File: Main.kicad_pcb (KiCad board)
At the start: 2 copper layers, 170.2 x 137.2 mm, 60 parts, among them J1 Conn_01x01_Male, J2 Conn_01x06_Male, J3 Conn_01x04_Male, J4 Conn_01x01_Male, J5 Conn_01x05_Male, J6 Conn_01x03, J7 Conn_01x03, J8 Conn_01x06, J9 Conn_01x05_Male, Q1 CSD17307Q5A, Q2 CSD17307Q5A, U1 LM4120-CustomSymbols, U2 LTC2942, U3 LM393, U4 TPS2557, U5 LM393, U6 TPS2557, U7 SN74LVC2G08

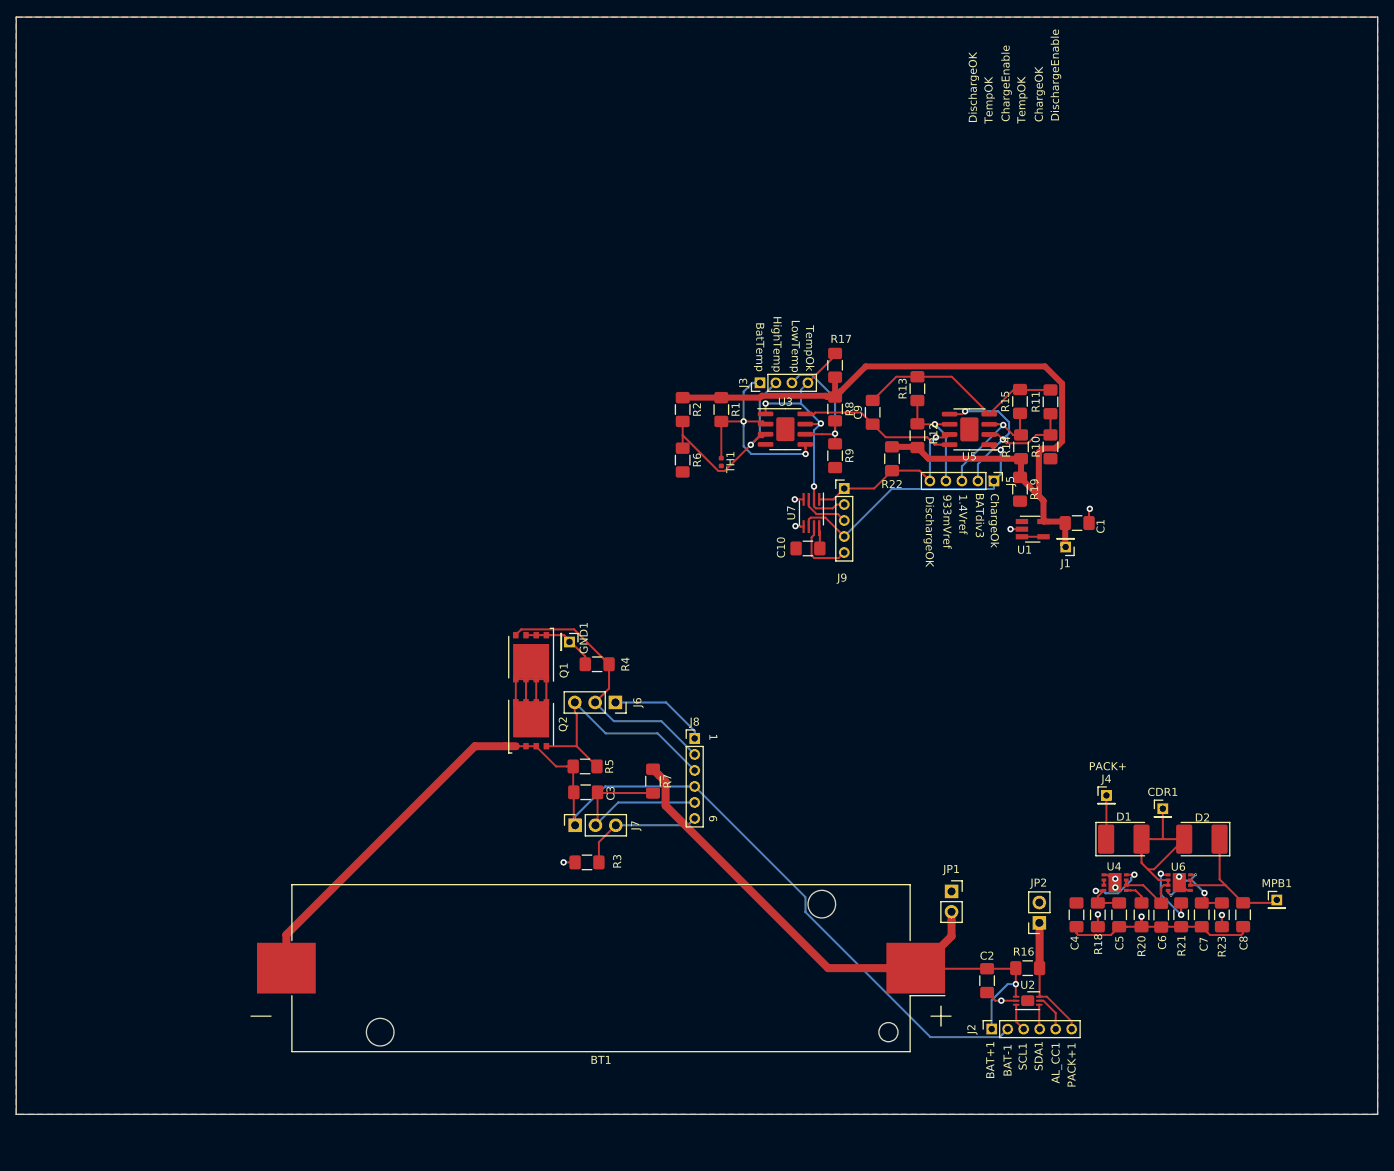
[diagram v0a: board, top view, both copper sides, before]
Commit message: progress
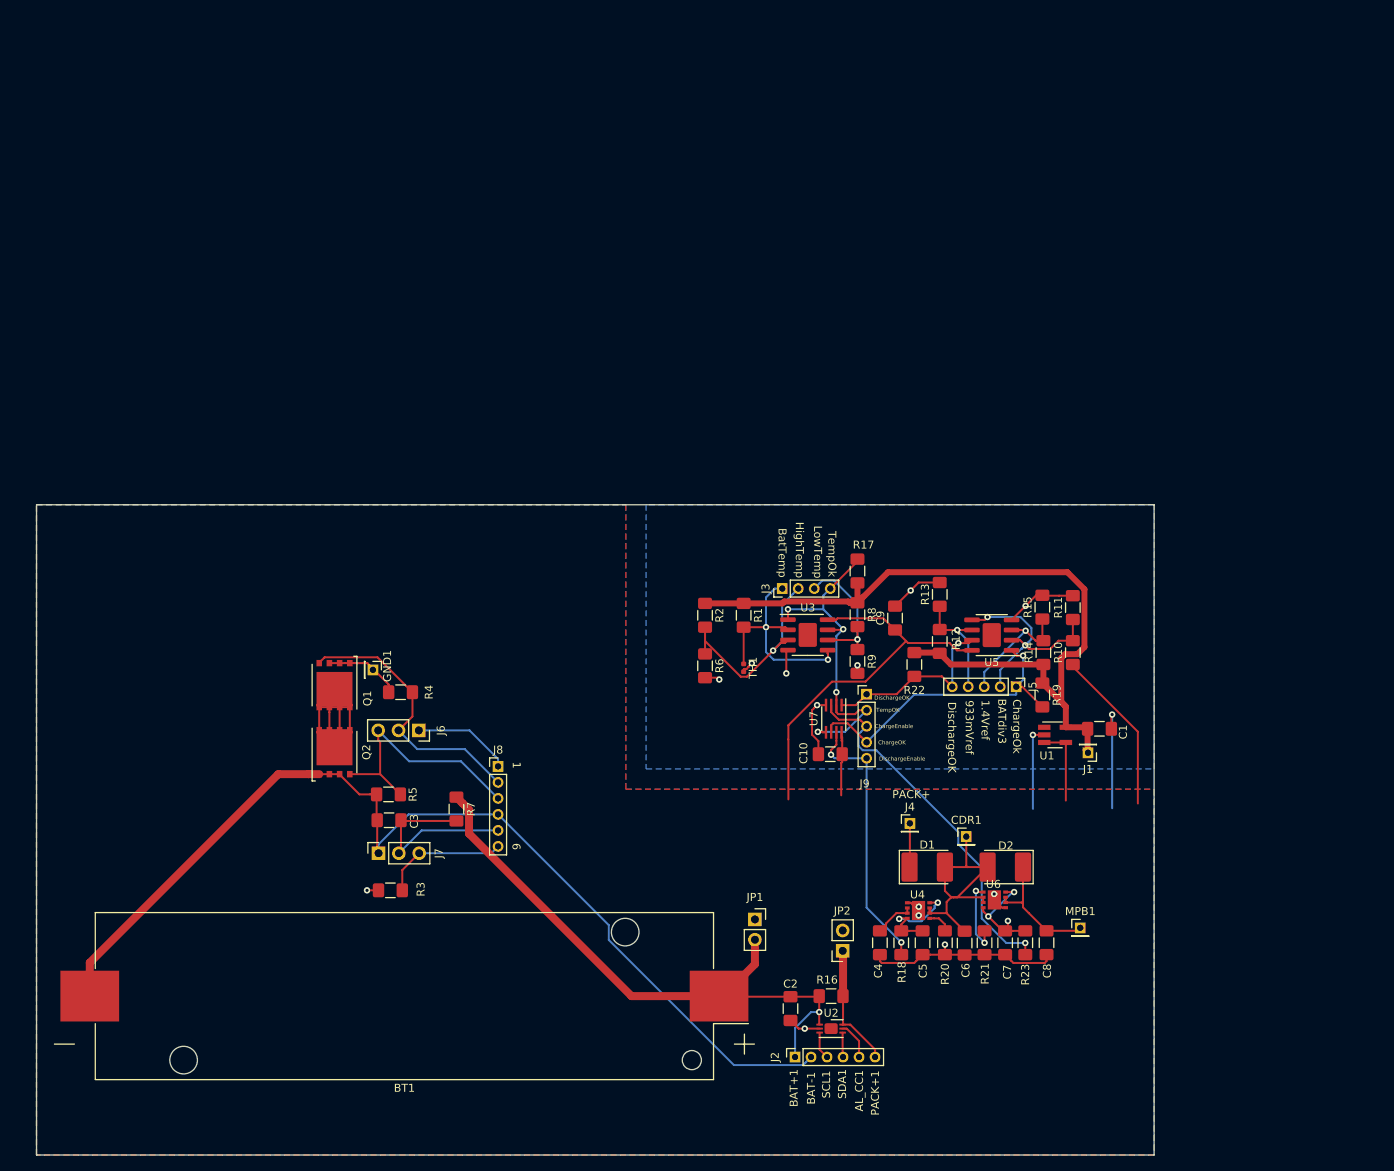
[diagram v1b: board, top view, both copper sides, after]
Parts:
- moved C1 25.9 mm to (160.8, 109.3)
- moved C10 25.9 mm to (127.2, 112.5)
- moved J5 25.9 mm to (150.4, 104.0)
- moved J9 25.9 mm to (131.7, 105.0)
- moved R1 25.9 mm to (116.3, 95.1)
- moved R14 25.9 mm to (153.8, 99.8)
- moved R17 25.9 mm to (130.6, 89.6)
- moved R2 25.9 mm to (111.5, 95.1)
- moved R22 25.9 mm to (137.7, 101.2)
- moved R6 25.9 mm to (111.5, 101.4)
- moved R8 25.9 mm to (130.6, 95.0)
- moved R9 25.9 mm to (130.6, 100.9)
- moved TH1 25.9 mm to (116.3, 101.7)
- moved U3 25.9 mm to (124.3, 97.5)
- moved U5 25.9 mm to (147.3, 97.6)
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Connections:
- U7 pad 4: GNDD -> GNDA
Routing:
- net PACK+: track 31.9 -> 97.9 mm
- net ChargeEnable: track 7.49 -> 46.0 mm
- net DischargeEnable: track 9.78 -> 34.1 mm, vias 1 -> 2
- net GNDD: track 47.9 -> 67.6 mm, vias 9 -> 8
- net TempOK: track 34.6 -> 41.8 mm
- net GNDA: track 26.7 -> 31.3 mm, vias 0 -> 7
- net ChargeOK: track 35.3 -> 39.6 mm
- net MPB: track 18.6 -> 16.4 mm
- net Net-(C7-Pad1): track 12.0 -> 13.7 mm
- net Net-(R21-Pad1): track 8.65 -> 9.38 mm
- added copper zone on B.Cu, net GNDA
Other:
- board size 170.2 x 137.2 mm -> 139.7 x 81.3 mm
